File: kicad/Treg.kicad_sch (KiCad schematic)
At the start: 31 parts, among them U1 PMW3360, U2 TPS73601DBV, U4 XIAO-ESP32-S3-DIP

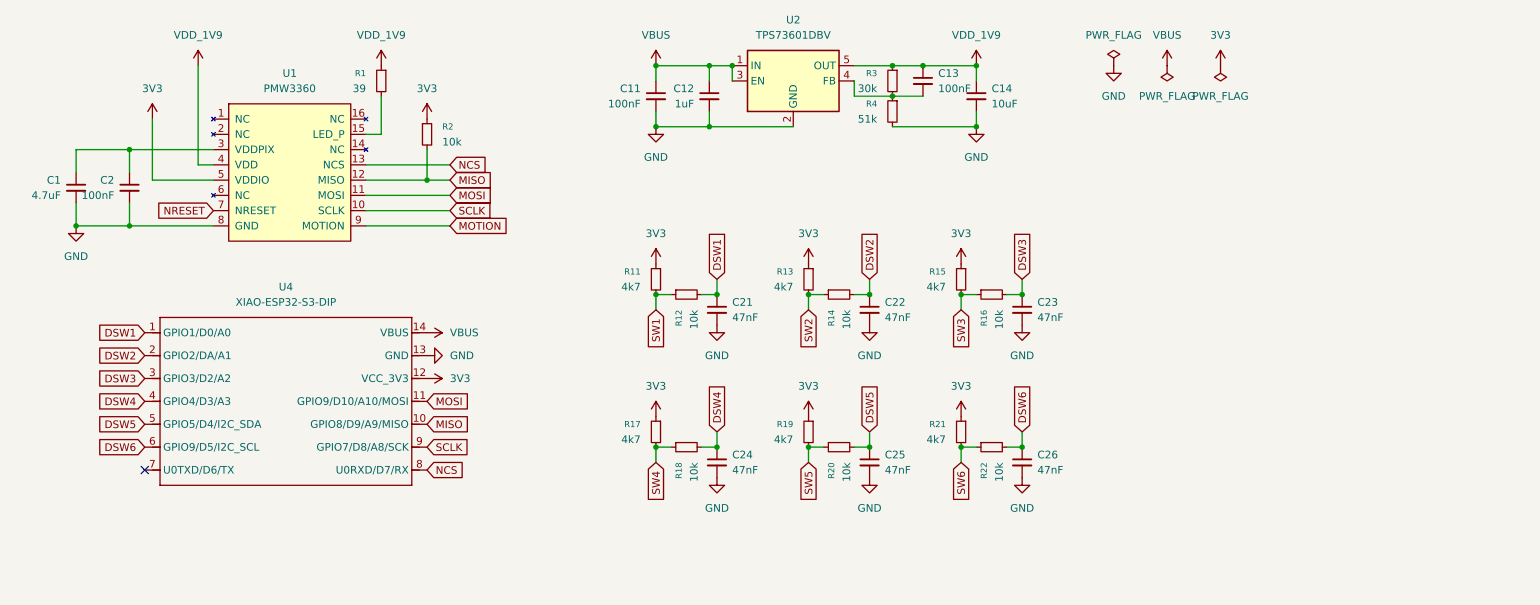
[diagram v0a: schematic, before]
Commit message: adjust layout
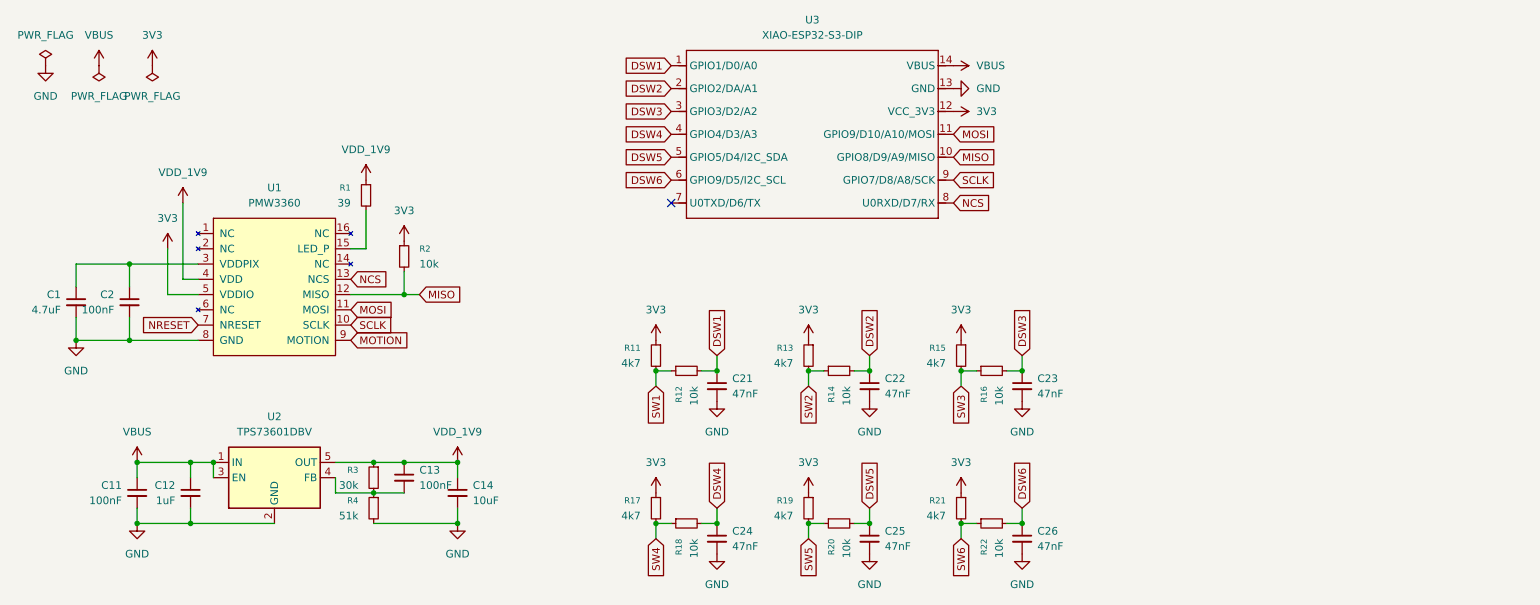
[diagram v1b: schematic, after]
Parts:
- renumbered U4 to U3
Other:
- moved on the sheet: C1, C11, C12, C13, C14, C2, C21, C22, C23, C24, C25, C26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

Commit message: add python
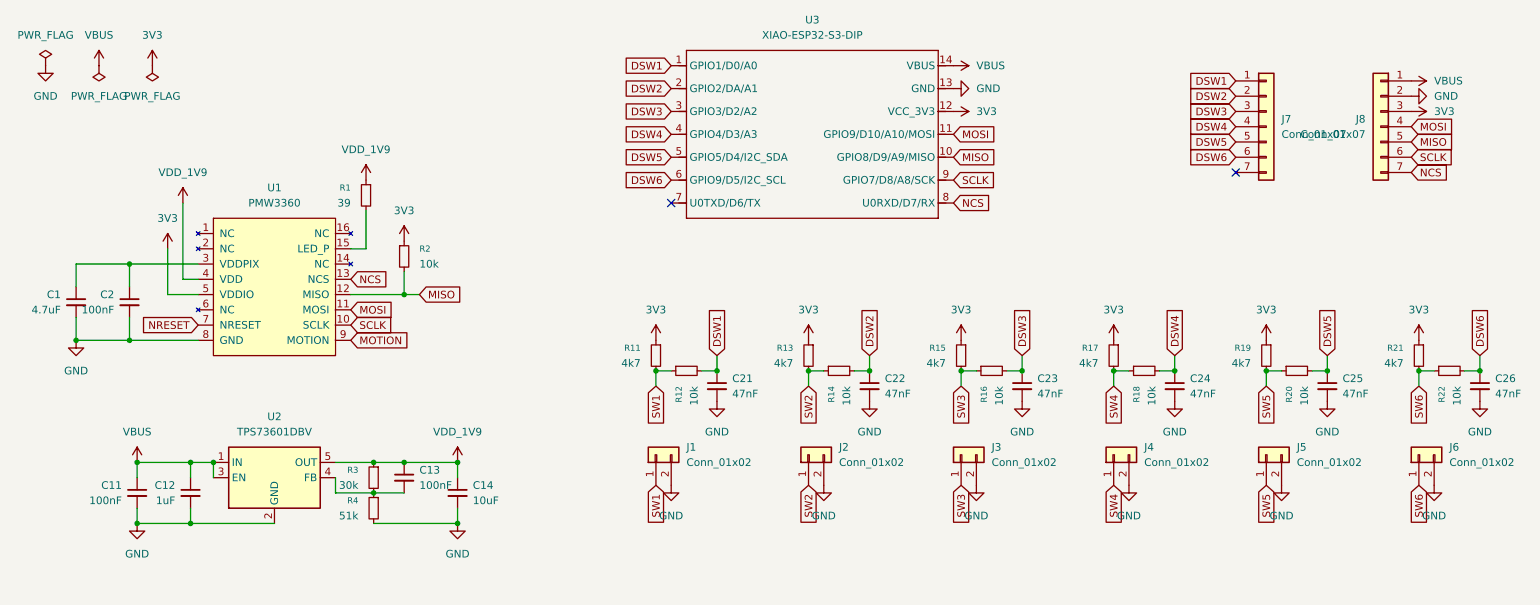
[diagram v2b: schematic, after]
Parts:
- added J1, J2, J3, J4, J5, J6: Conn_01x02, Connector_PinHeader_2.54mm:PinHeader_1x02_P2.54mm_Vertical, symbol Connector_Generic:Conn_01x02
- added J7, J8: Conn_01x07, Connector_PinHeader_2.54mm:PinHeader_1x07_P2.54mm_Vertical, symbol Connector_Generic:Conn_01x07
- C1, C11, C12, C13, C14, C2, C21, C22, C23, C24, C25, C26: footprint (none) -> Capacitor_SMD:C_0603_1608Metric_Pad1.08x0.95mm_HandSolder
- R1, R11, R12, R13, R14, R15, R16, R17, R18, R19, R2, R20, R21, R22, R3, R4: footprint (none) -> Resistor_SMD:R_0603_1608Metric_Pad0.98x0.95mm_HandSolder
- U1: footprint (none) -> PMW3360:PMW3360
- U2: footprint Package_TO_SOT_SMD:SOT-23-5 -> Package_TO_SOT_SMD:TSOT-23-5_HandSoldering
- U3: footprint Module:MOUDLE14P-XIAO-DIP-SMD -> RF_Module:MCU_Seeed_ESP32C3
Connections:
- net 3V3: now also J8.3 (Pin_3)
- net DSW1: now also J7.1 (Pin_1)
- net DSW2: now also J7.2 (Pin_2)
- net DSW3: now also J7.3 (Pin_3)
- net DSW4: now also J7.4 (Pin_4)
- net DSW5: now also J7.5 (Pin_5)
- net DSW6: now also J7.6 (Pin_6)
- net GND: now also J1.2 (Pin_2), J2.2 (Pin_2), J3.2 (Pin_2), J4.2 (Pin_2), J5.2 (Pin_2), J6.2 (Pin_2), J8.2 (Pin_2)
- net MISO: now also J8.5 (Pin_5)
- net MOSI: now also J8.4 (Pin_4)
- net NCS: now also J8.7 (Pin_7)
- net SCLK: now also J8.6 (Pin_6)
- net SW1: now also J1.1 (Pin_1)
- net SW2: now also J2.1 (Pin_1)
- net SW3: now also J3.1 (Pin_1)
- net SW4: now also J4.1 (Pin_1)
- net SW5: now also J5.1 (Pin_1)
- net SW6: now also J6.1 (Pin_1)
- net VBUS: now also J8.1 (Pin_1)
- no-connect marks 1 -> 2
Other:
- moved on the sheet: C24, C25, C26, R17, R18, R19, R20, R21, R22
